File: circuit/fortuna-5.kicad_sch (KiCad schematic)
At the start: 21 parts, among them J1 Debug, J2 Conn_01x08, SW1 SW_Push, SW4 CLOCK, U1 ATmega2560-16C, U2 Z80CPU, U3 AS6C4008-55PCN, U4 74HC04, U5 74LS32, U6 74HC00, U7 74HC14, Y1 20Mhz

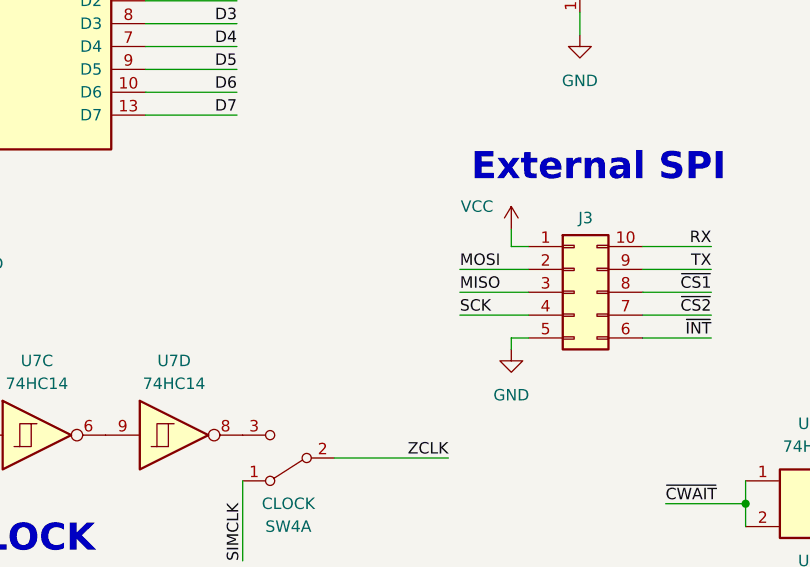
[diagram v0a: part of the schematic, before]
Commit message: .
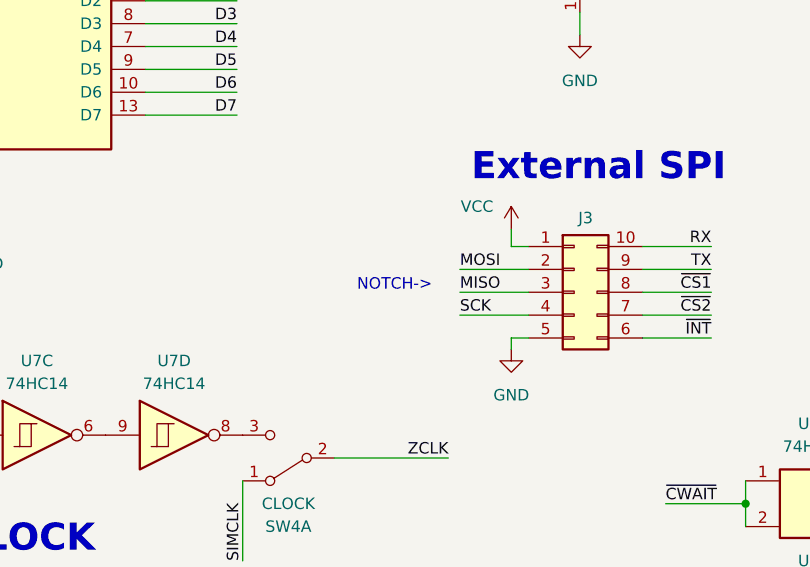
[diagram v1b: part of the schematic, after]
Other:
- note added: "NOTCH->"
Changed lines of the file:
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@@
     (effects (font (size 3 3) (thickness 0.6) bold) (justify left bottom))
+  )
+  (text "NOTCH->" (at 177.165 123.19 0)
+    (effects (font (size 1.27 1.27)) (justify left bottom))
   )
   (text "External SPI" (at 189.865 111.125 0)
